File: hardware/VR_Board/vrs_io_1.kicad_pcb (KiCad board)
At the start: 2 copper layers, 38.1 x 12.7 mm, 38 parts, among them U101 MAX9926/9927

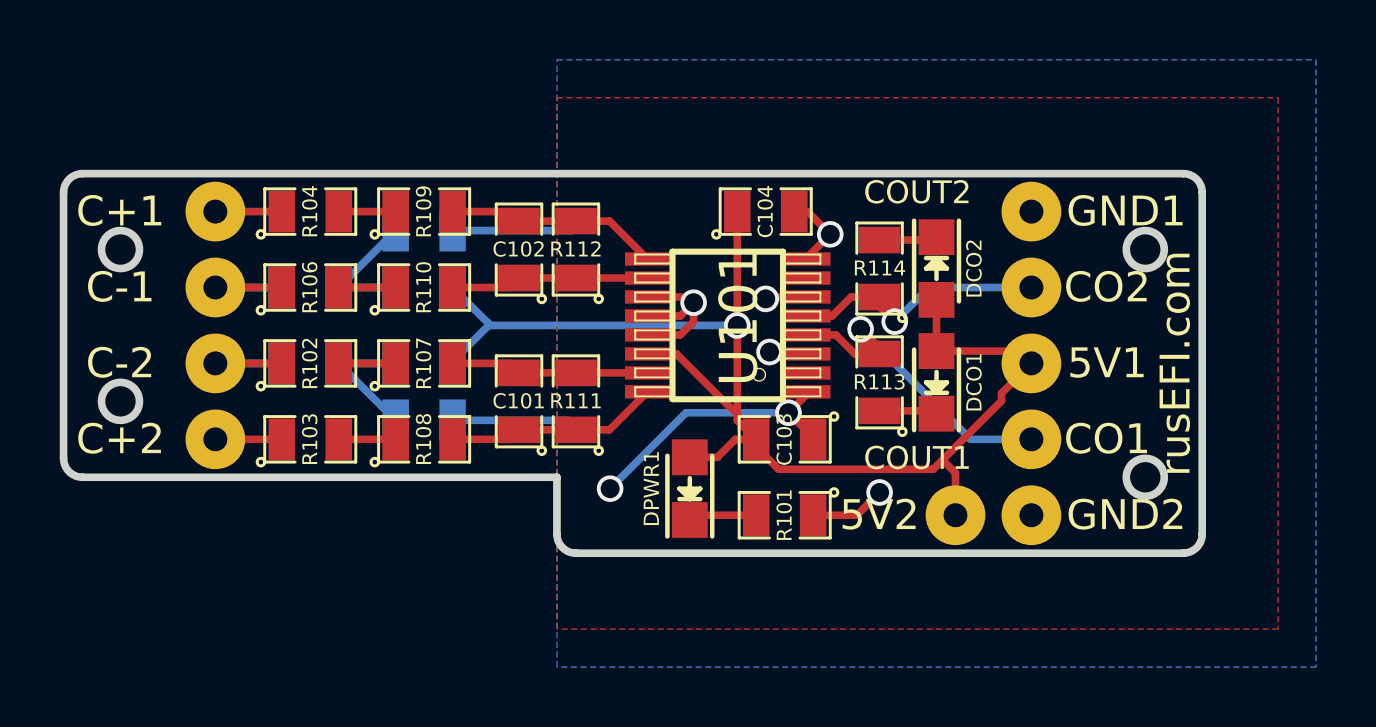
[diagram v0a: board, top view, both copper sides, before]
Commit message: update pcb files
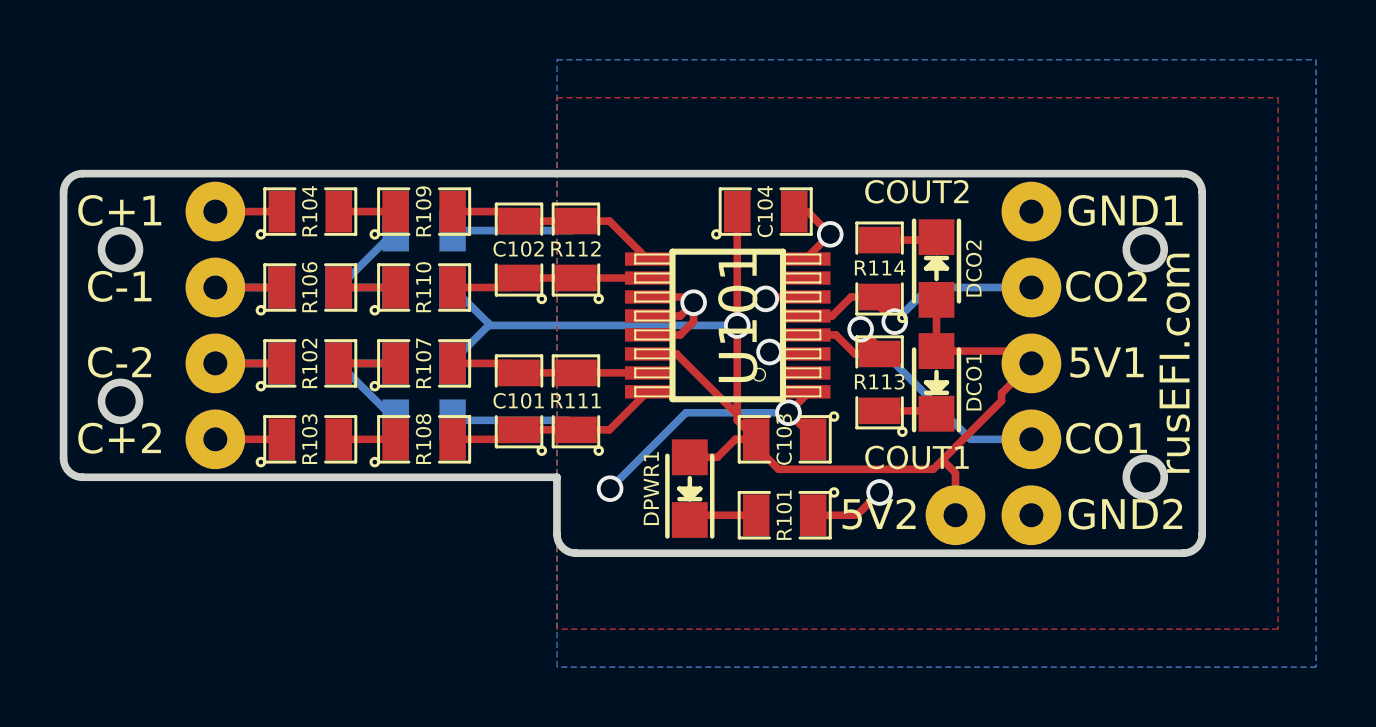
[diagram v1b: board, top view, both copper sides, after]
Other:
- net class Default removed
